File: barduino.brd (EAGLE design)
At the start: 54.9 x 47.4 mm, 28 parts, among them Q1 16MHz

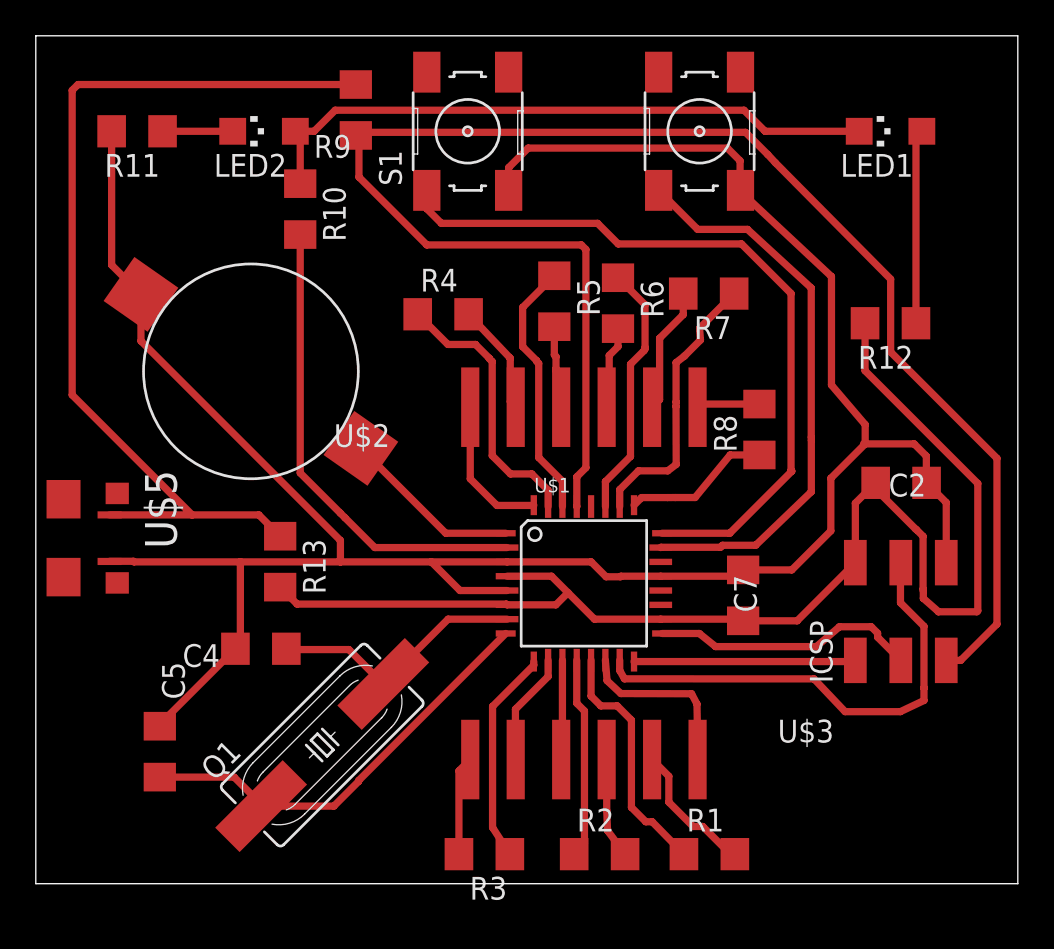
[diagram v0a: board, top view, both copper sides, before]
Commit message: only a couple air wires left
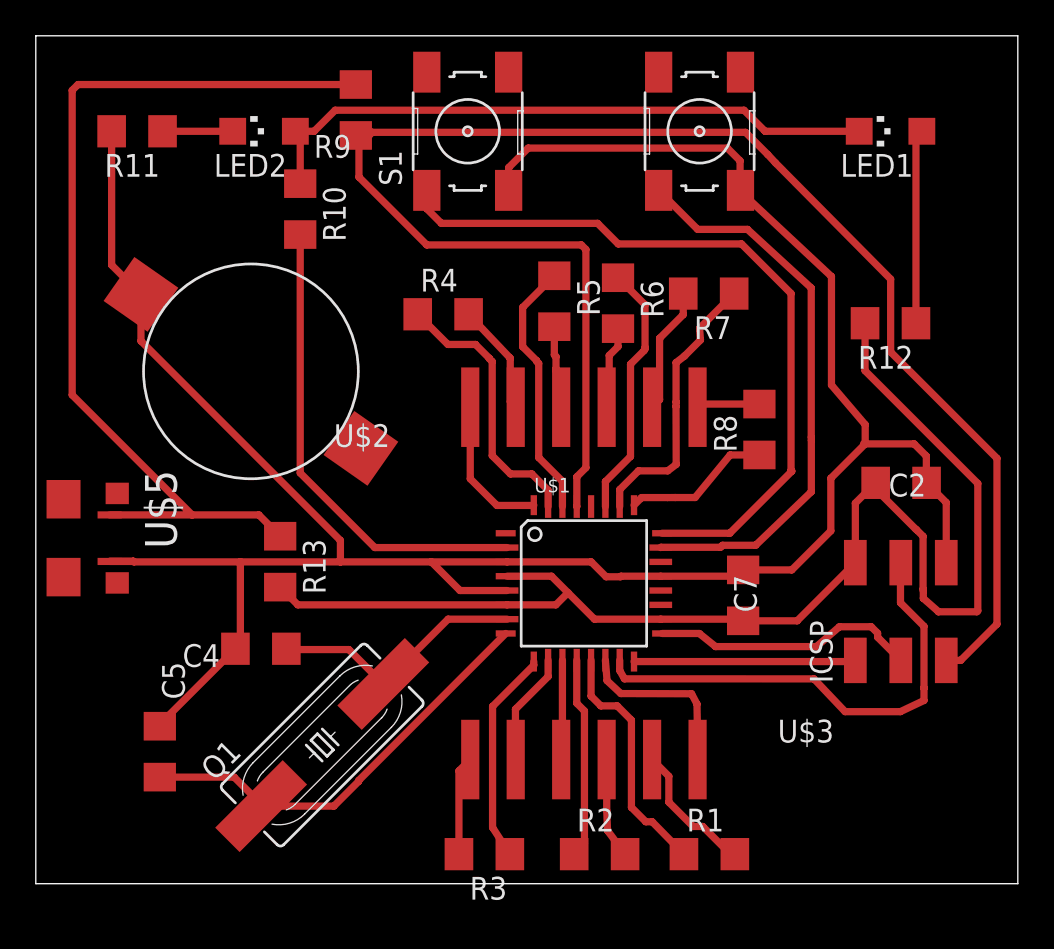
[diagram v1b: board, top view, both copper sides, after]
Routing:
- net D3: track 10.1 -> 0.00 mm
- net GND: track 137.3 -> 138.8 mm
- net RESET: track 90.2 -> 91.4 mm
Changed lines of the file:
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@@
 <setting verticaltext="up"/>
 </settings>
-<grid distance="0.01" unitdist="inch" unit="inch" style="lines" multiple="1" display="no" altdistance="0.025" altunitdist="inch" altunit="inch"/>
+<grid distance="0.0001" unitdist="inch" unit="inch" style="lines" multiple="1" display="no" altdistance="0.025" altunitdist="inch" altunit="inch"/>
 <layers>
 <layer number="1" name="Top" color="12" fill="1" visible="yes" active="yes"/>
@@
 <wire x1="26.518" y1="40.97741875" x2="32.8168" y2="34.67861875" width="0.4064" layer="1"/>
 <contactref element="R13" pad="1"/>
-<wire x1="6.5177" y1="27.8983" x2="6.476" y2="27.94" width="0.4064" layer="1"/>
 <contactref element="U$5" pad="VBUS"/>
 <contactref element="R13" pad="2"/>
-<wire x1="-5.21168125" y1="27.94" x2="-6.1595" y2="28.88781875" width="0.4064" layer="1"/>
-<wire x1="6.476" y1="27.94" x2="-5.21168125" y2="27.94" width="0.4064" layer="1"/>
 <wire x1="-15.687" y1="32.923" x2="-11.079" y2="32.923" width="0.4064" layer="1"/>
 <wire x1="-11.079" y1="32.923" x2="-7.35068125" y2="32.923" width="0.4064" layer="1"/>
@@
 <wire x1="-7.35068125" y1="32.923" x2="-6.1595" y2="31.73181875" width="0.4064" layer="1"/>
 <wire x1="-17.455271875" y1="56.966728125" x2="-1.932884375" y2="56.966728125" width="0.4064" layer="1"/>
-<wire x1="-1.932884375" y1="56.966728125" x2="-1.93288125" y2="56.96673125" width="0" layer="19" extent="1-1"/>
-<wire x1="-6.1595" y1="28.88781875" x2="-6.1595" y2="31.73181875" width="0" layer="19" extent="1-1"/>
+<wire x1="-1.932884375" y1="56.966728125" x2="-1.93288125" y2="56.96673125" width="0.635" layer="1"/>
+<wire x1="-1.82245" y1="57.01665" x2="-1.932884375" y2="56.966728125" width="0.635" layer="1"/>
+<wire x1="6.5177" y1="27.8983" x2="-5.16998125" y2="27.8983" width="0.4064" layer="1"/>
+<wire x1="-5.16998125" y1="27.8983" x2="-6.1595" y2="28.88781875" width="0.4064" layer="1"/>
+<wire x1="-6.1595" y1="31.73181875" x2="-6.1595" y2="28.88781875" width="0" layer="19" extent="1-1"/>
 </signal>
 <signal name="GND" class="1">
@@
 <wire x1="-12.628825" y1="21.47535625" x2="-12.882825" y2="21.47535625" width="0.4064" layer="1"/>
 <wire x1="-8.382" y1="30.2983" x2="-14.32519375" y2="30.2983" width="0.4064" layer="1"/>
-<wire x1="-14.32519375" y1="30.2983" x2="-14.35949375" y2="30.3326" width="0.4064" layer="1"/>
 <wire x1="-14.35949375" y1="30.3326" x2="-15.687" y2="30.3326" width="0.4064" layer="1"/>
 <wire x1="-2.794" y1="30.2983" x2="-2.794" y2="31.496" width="0.4064" layer="1"/>
 <wire x1="-15.71435625" y1="54.216525" x2="-15.57488125" y2="54.356" width="0.4064" layer="1"/>
-<wire x1="-2.794" y1="31.496" x2="-13.93635625" y2="42.63835625" width="0.4064" layer="1"/>
-<wire x1="-13.93635625" y1="42.63835625" x2="-13.93635625" y2="45.24408125" width="0.4064" layer="1"/>
+<wire x1="6.5177" y1="28.6983" x2="3.886" y2="28.6983" width="0.4064" layer="1"/>
+<wire x1="3.886" y1="28.6983" x2="2.286" y2="30.2983" width="0.4064" layer="1"/>
 <wire x1="-15.57488125" y1="54.356" x2="-15.57488125" y2="46.88260625" width="0.4064" layer="1"/>
 <wire x1="-15.57488125" y1="46.88260625" x2="-13.93635625" y2="45.24408125" width="0.4064" layer="1"/>
-<wire x1="6.5177" y1="28.6983" x2="3.886" y2="28.6983" width="0.4064" layer="1"/>
-<wire x1="3.886" y1="28.6983" x2="2.286" y2="30.2983" width="0.4064" layer="1"/>
-<wire x1="-13.93635625" y1="45.24408125" x2="-13.93635625" y2="45.244084375" width="0" layer="19" extent="1-1"/>
-<wire x1="-15.687" y1="30.323" x2="-15.687" y2="30.3326" width="0" layer="19" extent="1-1"/>
+<wire x1="-13.93635625" y1="42.63835625" x2="-2.794" y2="31.496" width="0.4064" layer="1"/>
+<wire x1="-13.93635625" y1="45.24408125" x2="-13.93635625" y2="42.63835625" width="0.4064" layer="1"/>
+<wire x1="-15.687" y1="30.323" x2="-14.36909375" y2="30.323" width="0.4064" layer="1"/>
+<wire x1="-14.36909375" y1="30.323" x2="-14.35949375" y2="30.3326" width="0.4064" layer="1"/>
+<wire x1="-14.32519375" y1="30.2983" x2="-14.35949375" y2="30.3326" width="0.4064" layer="1"/>
+<wire x1="-13.93635625" y1="45.24408125" x2="-13.93635625" y2="45.244084375" width="0.635" layer="1"/>
+<wire x1="-13.79855" y1="45.3009" x2="-13.93635625" y2="45.24408125" width="0.635" layer="1"/>
 </signal>
 <signal name="PB7">
@@
 <wire x1="21.07691875" y1="53.0606" x2="21.50871875" y2="52.59578125" width="0.4064" layer="1"/>
 <wire x1="27.947621875" y1="46.09591875" x2="21.50871875" y2="52.59578125" width="0.4064" layer="1"/>
-<wire x1="19.8399375" y1="54.29758125" x2="-1.7580375" y2="54.29758125" width="0.4064" layer="1"/>
-<wire x1="-1.7580375" y1="54.29758125" x2="-1.93288125" y2="54.1227375" width="0.4064" layer="1"/>
+<wire x1="19.8399375" y1="54.29758125" x2="-1.016" y2="54.29758125" width="0.4064" layer="1"/>
+<wire x1="-1.016" y1="54.29758125" x2="-1.7580375" y2="54.29758125" width="0.4064" layer="1"/>
 <wire x1="33.886440625" y1="36.08548125" x2="27.947621875" y2="42.0243" width="0.4064" layer="1"/>
 <wire x1="27.947621875" y1="42.0243" x2="27.947621875" y2="46.09591875" width="0.4064" layer="1"/>
@@
 <wire x1="10.668" y1="48.006" x2="2.032" y2="48.006" width="0.4064" layer="1"/>
 <wire x1="2.032" y1="48.006" x2="-1.7580375" y2="51.7960375" width="0.4064" layer="1"/>
-<wire x1="-1.7580375" y1="51.7960375" x2="-1.7580375" y2="54.29758125" width="0.4064" layer="1"/>
+<wire x1="-1.7580375" y1="51.7960375" x2="-1.7580375" y2="54.1528" width="0.4064" layer="1"/>
+<wire x1="-1.7580375" y1="54.1528" x2="-1.7580375" y2="54.29758125" width="0.4064" layer="1"/>
 <wire x1="10.922" y1="35.56" x2="10.922" y2="47.752" width="0.4064" layer="1"/>
-<wire x1="-1.93288125" y1="54.1227375" x2="-1.93288125" y2="54.12273125" width="0" layer="19" extent="1-1"/>
+<wire x1="-1.93288125" y1="54.1227375" x2="-1.7580375" y2="54.29758125" width="0.4064" layer="1"/>
+<wire x1="-1.93288125" y1="54.1227375" x2="-1.19084375" y2="54.1227375" width="0.4064" layer="1"/>
+<wire x1="-1.19084375" y1="54.1227375" x2="-1.016" y2="54.29758125" width="0.4064" layer="1"/>
+<wire x1="-1.82245" y1="54.1528" x2="-1.93288125" y2="54.12273125" width="0.635" layer="1"/>
+<wire x1="-1.82245" y1="54.1528" x2="-1.7580375" y2="54.1528" width="0.635" layer="1"/>
 </signal>
 <signal name="PB6">
@@
 <contactref element="U$1" pad="1"/>
 <contactref element="U$4" pad="P$1"/>
-<wire x1="6.4415" y1="31.8983" x2="3.09305625" y2="31.8983" width="0.4064" layer="1"/>
-<wire x1="3.09305625" y1="31.8983" x2="-1.649078125" y2="36.640434375" width="0.4064" layer="1"/>
-<wire x1="-1.649078125" y1="36.640434375" x2="-1.649078125" y2="36.6404375" width="0" layer="19" extent="1-1"/>
+<wire x1="-1.649078125" y1="36.6404375" x2="6.4415" y2="31.8983" width="0" layer="19" extent="1-1"/>
 </signal>
 <signal name="D4">
@@
 <contactref element="R10" pad="2"/>
 <wire x1="6.5177" y1="31.0983" x2="-0.8723" y2="31.0983" width="0.4064" layer="1"/>
-<wire x1="-0.8723" y1="31.0983" x2="-2.54" y2="32.766" width="0.4064" layer="1"/>
-<wire x1="-2.54" y1="32.766" x2="-2.794" y2="33.02" width="0.4064" layer="1"/>
-<wire x1="-2.794" y1="33.02" x2="-5.0393625" y2="35.2653625" width="0.4064" layer="1"/>
+<wire x1="-0.8723" y1="31.0983" x2="-5.0393625" y2="35.2653625" width="0.4064" layer="1"/>
 <wire x1="-5.0393625" y1="35.2653625" x2="-5.0393625" y2="48.585521875" width="0.4064" layer="1"/>
 </signal>
